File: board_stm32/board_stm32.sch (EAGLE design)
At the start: 8 parts, among them IC2 NE555, T1 BC547

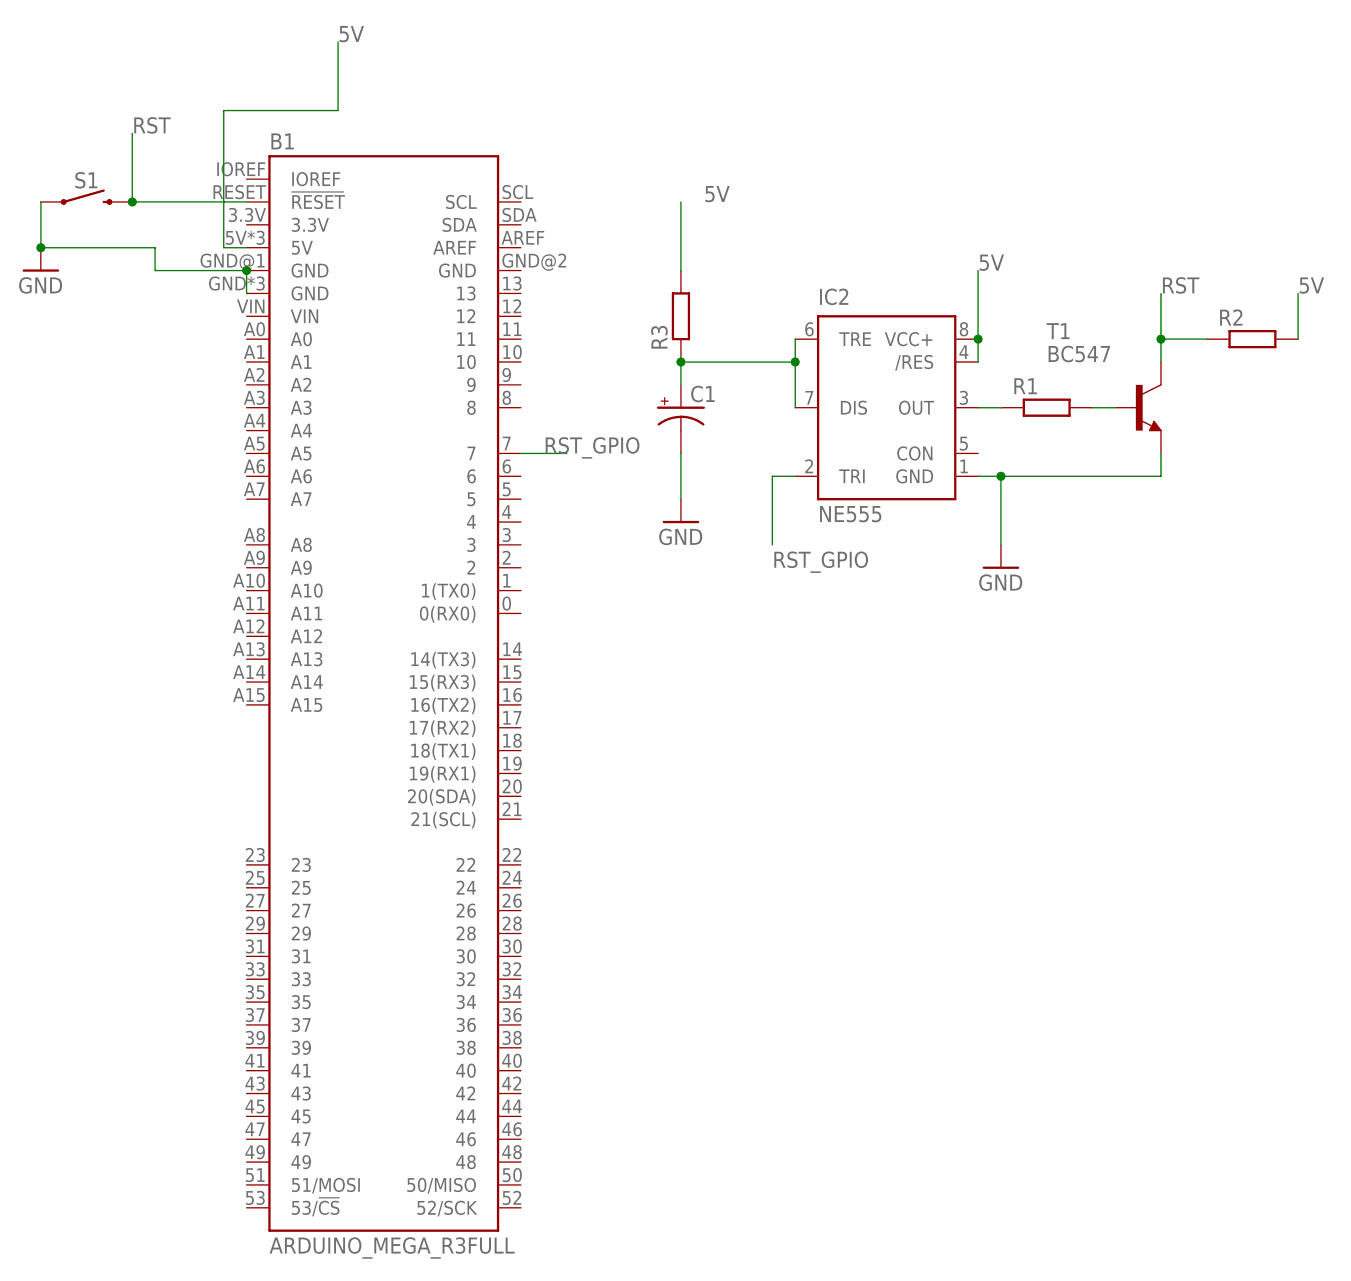
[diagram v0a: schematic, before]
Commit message: update schematic and board, add .gitignore
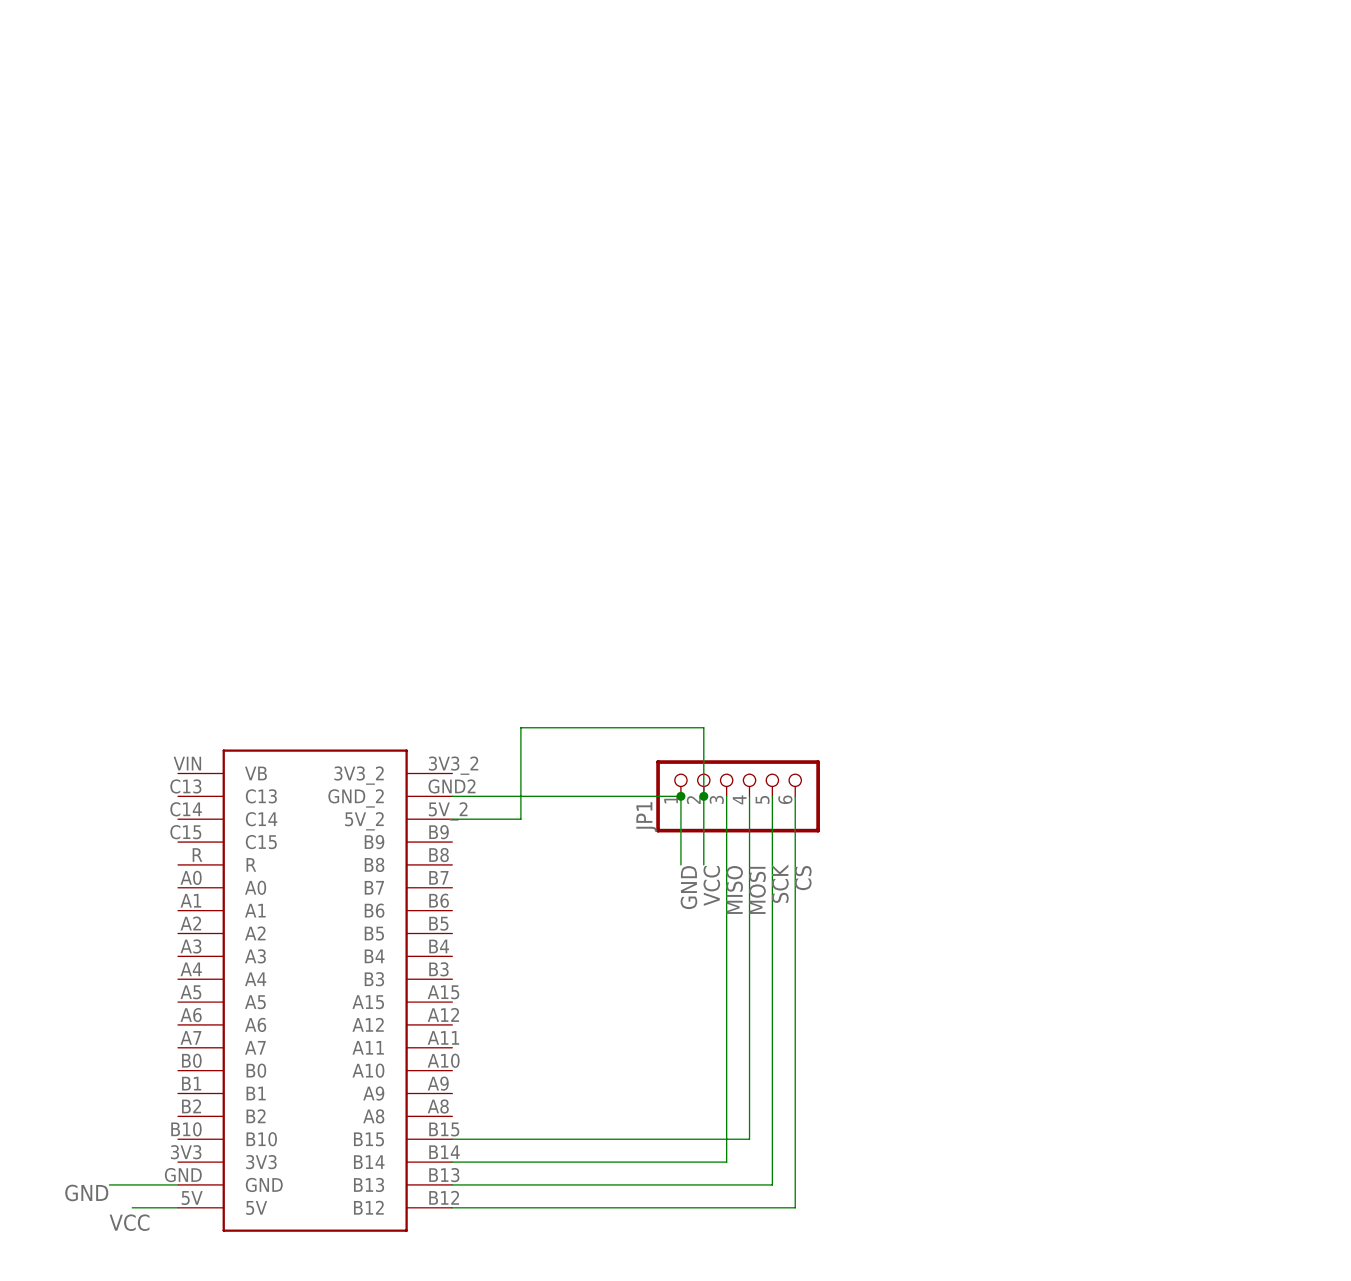
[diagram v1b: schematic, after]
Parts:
- removed B1: ARDUINO_MEGA_R3FULL, SparkFun-Boards:ARDUINO_MEGA_R3FULL
- removed C1: (no value), rcl:CPOL-USE2.5-6
- removed IC2: NE555, st-microelectronics:NE555
- removed R1, R2, R3: (no value), rcl:R-EU_0204/7
- removed S1: MOMENTARY-SWITCH-SPST-PTH-6.0MM, SparkFun-Switches:MOMENTARY-SWITCH-SPST-PTH-6.0MM
- removed T1: BC547, transistor:BC547
- added JP1: (no value), adafruit:PINHD-1X6
- added U$1: STM32F411CEU6, STM32F411CEU6:STM32F411CEU6
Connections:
- removed net 5V: B1.5V, IC2./RES, IC2.VCC+, R2.2, R3.2
- removed net N$1: C1.+, IC2.DIS, IC2.TRE, R3.1
- removed net N$2: IC2.OUT, R1.1
- removed net N$3: R1.2, T1.B
- removed net RST: B1.!RESET, R2.1, S1.2, T1.C
- removed net RST_GPIO: B1.7, IC2.TRI
- new net CS: JP1.6, U$1.B12
- new net MISO: JP1.3, U$1.B14
- new net MOSI: JP1.4, U$1.B15
- new net SCK: JP1.5, U$1.B13
- new net VCC: JP1.2, U$1.5V, U$1.5V_2
- net GND: now also JP1.1, U$1.GND, U$1.GND_2; no longer B1.GND, B1.GND@2, C1.-, IC2.GND, S1.1, T1.E
